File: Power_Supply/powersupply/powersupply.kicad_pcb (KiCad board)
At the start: 2 copper layers, 54 parts, among them J1 Conn_01x03, J2 USB_B_Micro, Q1 Q_PMOS_GDS, SW1 SW_Push, U1 AZ1117E-3.3, U10 MCP6001-OT, U2 ATSAMD10D13A-SS, U3 B0505S-2WR2, U4 TFT_OLED, U5 joystick-K1-1506DN-01, U6 MC33063AP1, U7 LM358P, U8 1x2, U9 1x2

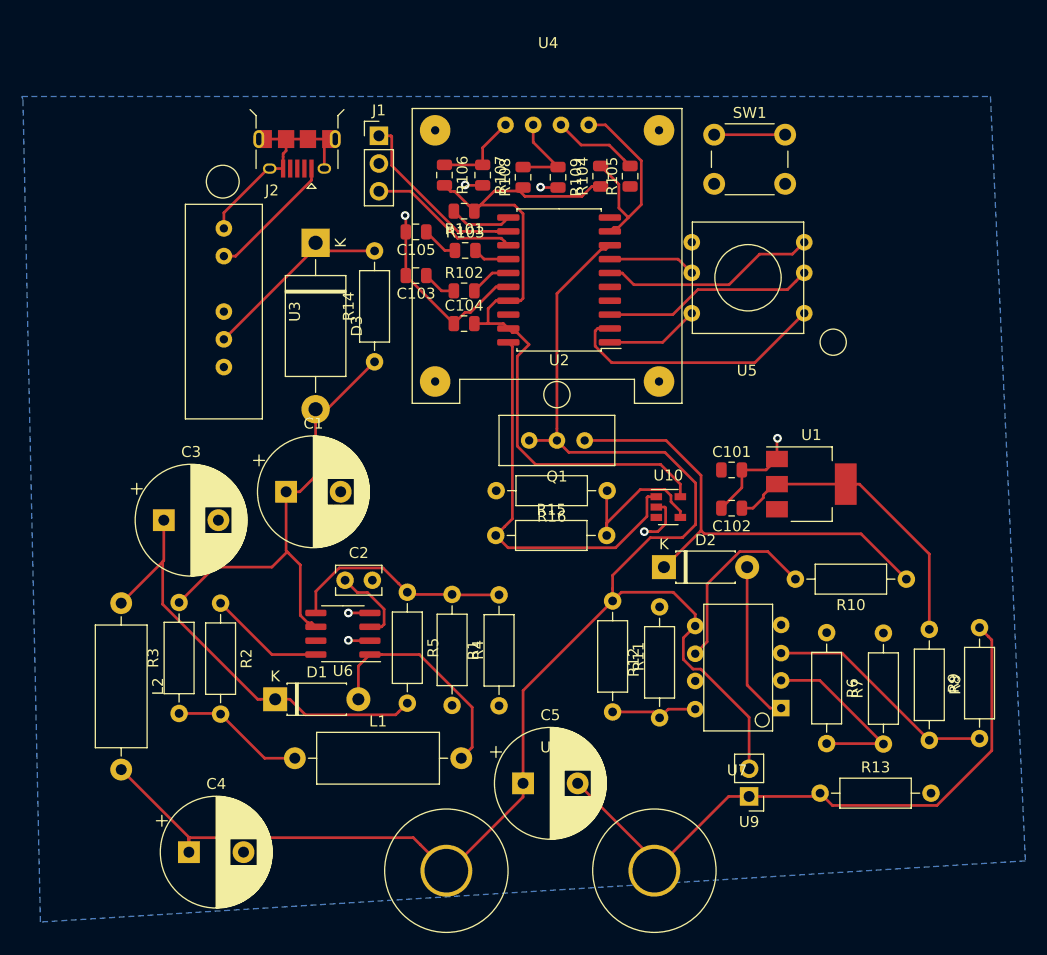
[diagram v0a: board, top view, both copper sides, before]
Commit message: layout changes
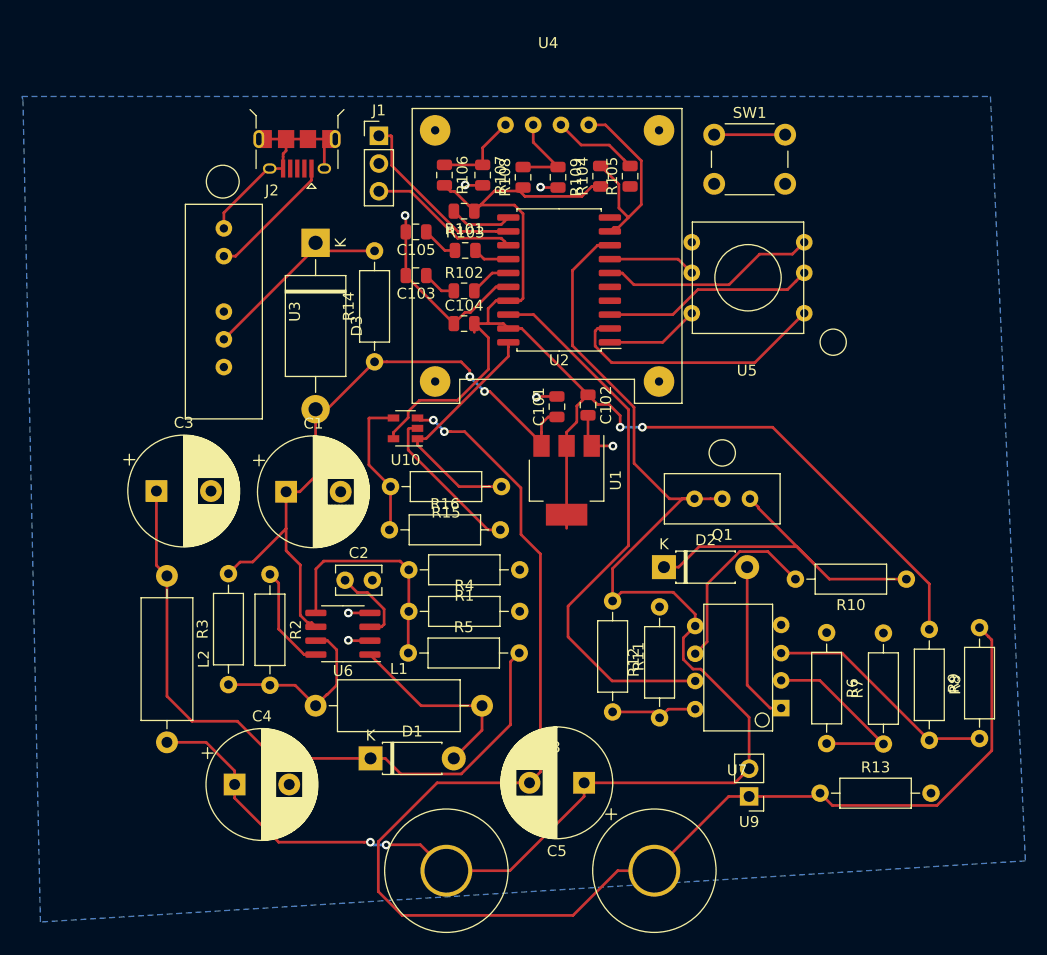
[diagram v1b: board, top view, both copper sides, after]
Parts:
- moved U10 25.1 mm to (75.1, 50.2), turned to 180 degrees
- moved U1 22.4 mm to (89.9, 54.9), turned to 270 degrees
- moved R16 20.3 mm to (73.7, 59.5), turned to 0 degrees
- moved C101 17.0 mm to (89.0, 48.2), turned to 90 degrees
- moved C102 16.2 mm to (91.8, 48.1), turned to 270 degrees
- moved Q1 16.1 mm to (104.1, 56.6)
- moved R1 12.6 mm to (85.6, 63.1), turned to 180 degrees
- moved D1 10.3 mm to (71.9, 80.4)
- moved C4 7.48 mm to (59.5, 82.8)
- moved C5 5.59 mm to (91.5, 82.7), turned to 180 degrees
- moved R5 5.57 mm to (75.4, 70.8), turned to 0 degrees
- moved R2 5.24 mm to (62.7, 63.6)
- moved R3 5.24 mm to (58.9, 73.7)
- moved L1 5.17 mm to (66.9, 75.6)
- moved L2 4.88 mm to (53.3, 63.7)
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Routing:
- net /V_negative_out: track 59.0 -> 137.0 mm, vias 0 -> 2
- net /V_lin_ctrl: track 0.00 -> 51.0 mm
- net +3V3: track 96.1 -> 122.2 mm, vias 0 -> 2
- net Net-(C3-Pad1): track 40.2 -> 62.4 mm
- net +5V: track 42.3 -> 60.0 mm, vias 0 -> 2
- net /V_current_amplified: track 36.6 -> 22.6 mm
- net Net-(D2-Pad1): track 42.5 -> 32.8 mm
- net /Boost_out: track 146.3 -> 137.4 mm, vias 0 -> 2
- net GND: track 39.9 -> 46.3 mm
- net Net-(L1-Pad1): track 12.3 -> 17.0 mm
- net Net-(D1-Pad2): track 21.0 -> 18.1 mm
- net Net-(R15-Pad2): track 15.0 -> 13.3 mm
- net Net-(R2-Pad1): track 10.7 -> 9.72 mm

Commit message: more layout
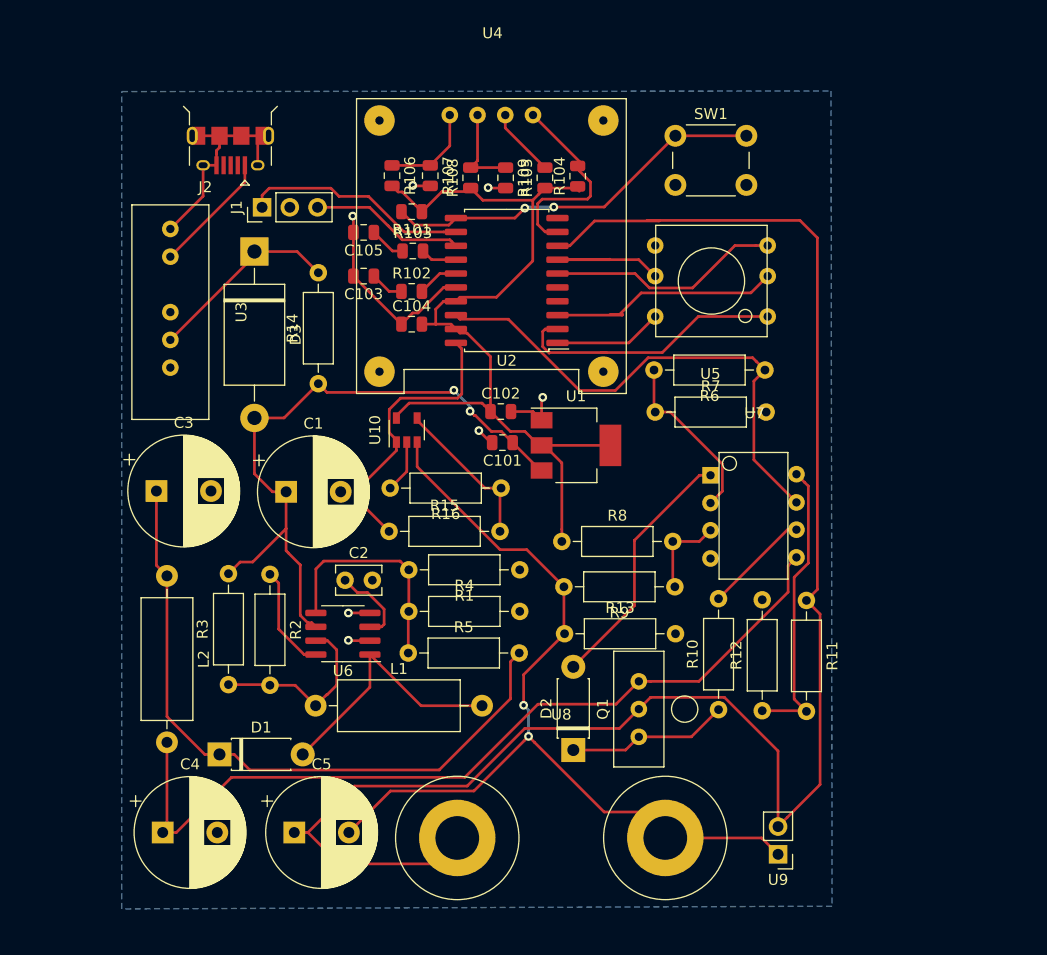
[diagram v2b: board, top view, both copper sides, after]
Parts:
- moved R7 36.9 mm to (98.0, 48.7), turned to 0 degrees
- moved R8 34.6 mm to (89.5, 60.5), turned to 0 degrees
- moved R9 31.2 mm to (99.8, 64.7), turned to 180 degrees
- moved R13 27.6 mm to (89.7, 69.0)
- moved C5 26.9 mm to (65.0, 87.2), turned to 0 degrees
- moved R6 24.7 mm to (108.0, 44.9), turned to 180 degrees
- moved R10 20.9 mm to (103.8, 76.0), turned to 90 degrees
- moved Q1 20.7 mm to (96.5, 75.9), turned to 90 degrees
- moved D2 18.7 mm to (90.5, 79.7), turned to 90 degrees
- moved R11 17.8 mm to (111.8, 66.0)
- moved U7 14.0 mm to (107.0, 58.2), turned to 0 degrees
- moved D1 13.8 mm to (58.1, 80.0)
- moved J1 12.5 mm to (62.0, 29.9), turned to 90 degrees
- moved R15 11.1 mm to (73.6, 59.6), turned to 0 degrees
- moved R16 10.9 mm to (83.9, 55.7), turned to 180 degrees
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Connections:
- C5 pad 1: /Boost_out -> /V_positive_out
- Q1 pad 2: /Boost_out -> /V_positive_out
- R11 pad 1: /Boost_out -> /V_positive_out
- R6 pad 1: /Vlim -> /V_lin_ctrl
- U2 pad 8: /Boost_out -> /V_positive_out
- U8 pad 2: /Boost_out -> /V_positive_out
- U9 pad 2: /Boost_out -> /V_positive_out
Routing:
- net /V_positive_out: track 0.00 -> 157.3 mm
- net /Boost_out: track 137.4 -> 78.3 mm, vias 2 -> 0
- net /V_negative_out: track 137.0 -> 83.2 mm
- net +3V3: track 122.2 -> 81.4 mm, vias 2 -> 0
- net Net-(R101-Pad2): track 12.3 -> 35.6 mm, vias 0 -> 2
- net Net-(R11-Pad2): track 8.12 -> 27.2 mm
- net Net-(D2-Pad1): track 32.8 -> 14.8 mm
- net Net-(R8-Pad2): track 21.5 -> 8.38 mm
- net GND: track 46.3 -> 37.1 mm
- net Net-(D2-Pad2): track 14.8 -> 23.3 mm
- net Net-(R10-Pad2): track 17.2 -> 9.75 mm
- net /right: track 8.02 -> 14.4 mm
- net Net-(D1-Pad2): track 18.1 -> 23.9 mm
- net /V_lin_ctrl: track 51.0 -> 47.0 mm
- net /SWCLK: track 17.0 -> 20.8 mm
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
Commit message: even more layout
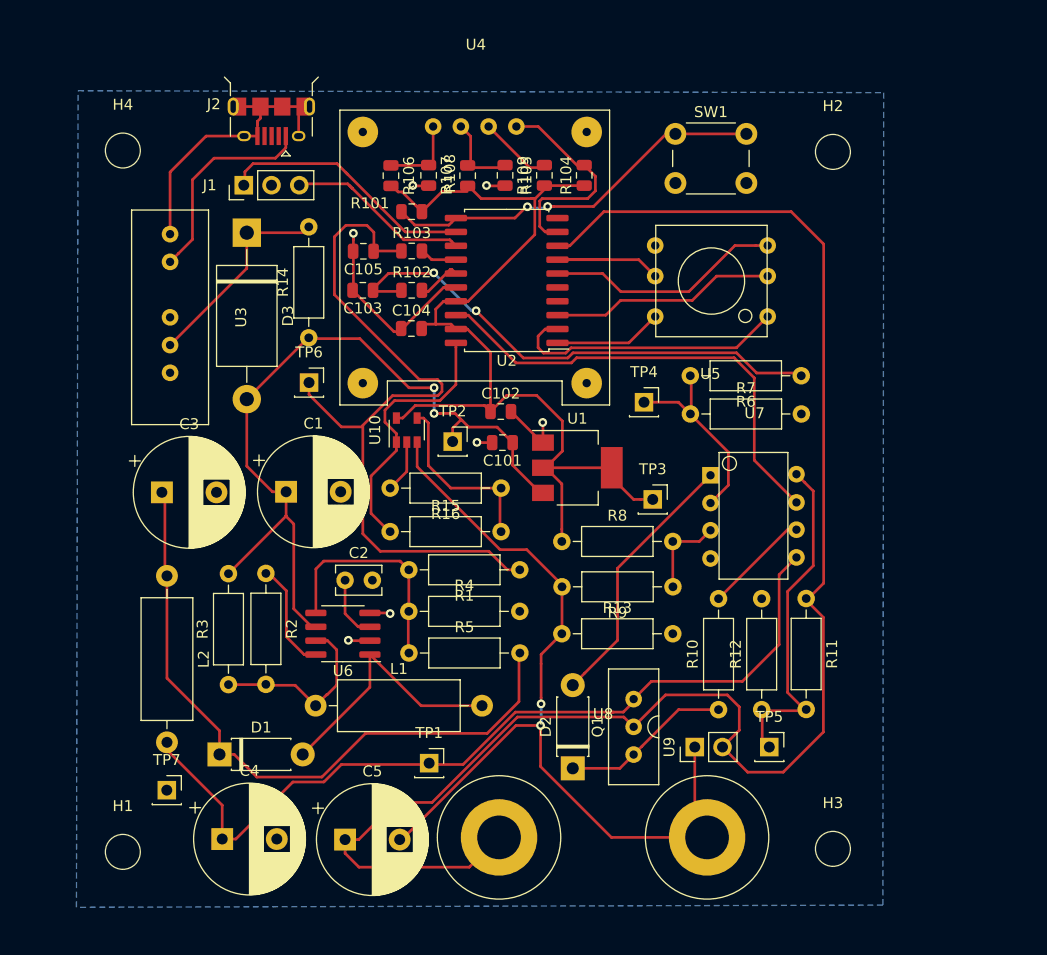
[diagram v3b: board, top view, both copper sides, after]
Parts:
- added H1: MountingHole, MountingHole:MountingHole_3.2mm_M3, F.Cu at (49.2, 89.0)
- added H2: MountingHole, MountingHole:MountingHole_3.2mm_M3, F.Cu at (114.3, 24.9)
- added H3: MountingHole, MountingHole:MountingHole_3.2mm_M3, F.Cu at (114.3, 88.7)
- added H4: MountingHole, MountingHole:MountingHole_3.2mm_M3, F.Cu at (49.2, 24.8)
- added TP1: Boost_out, Connector_PinSocket_2.54mm:PinSocket_1x01_P2.54mm_Vertical, F.Cu at (77.3, 80.8)
- added TP2: +5_isolated, Connector_PinSocket_2.54mm:PinSocket_1x01_P2.54mm_Vertical, F.Cu at (79.5, 51.4)
- added TP3: +3.3, Connector_PinSocket_2.54mm:PinSocket_1x01_P2.54mm_Vertical, F.Cu at (97.8, 56.7)
- added TP4: Current_limit, Connector_PinSocket_2.54mm:PinSocket_1x01_P2.54mm_Vertical, F.Cu at (97.0, 47.8)
- added TP5: Voltage_limit, Connector_PinSocket_2.54mm:PinSocket_1x01_P2.54mm_Vertical, F.Cu at (108.5, 79.4)
- added TP6: Boost_ctrl, Connector_PinSocket_2.54mm:PinSocket_1x01_P2.54mm_Vertical, F.Cu at (66.3, 46.0)
- added TP7: GND, Connector_PinSocket_2.54mm:PinSocket_1x01_P2.54mm_Vertical, F.Cu at (53.3, 83.3)
- moved U9 12.4 mm to (101.6, 79.4), turned to 90 degrees
- moved C4 5.48 mm to (58.4, 87.8)
- moved C5 4.70 mm to (69.6, 87.8)
- moved J2 4.61 mm to (62.9, 20.7)
- moved R14 4.29 mm to (66.3, 41.9)
- moved U8 3.83 mm to (93.2, 87.7)
- moved R6 3.37 mm to (111.4, 45.4)
- moved R7 3.23 mm to (101.2, 48.9)
- moved J1 2.63 mm to (60.3, 27.9)
- moved U1 2.05 mm to (90.9, 53.8)
- moved D3 1.86 mm to (60.6, 32.3)
- moved U4 1.85 mm to (81.5, 34.5)
- moved C105 1.73 mm to (71.3, 34.0)
- moved Q1 1.69 mm to (96.0, 77.5)
- moved D2 1.68 mm to (90.5, 81.3)
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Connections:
- net Net-(R11-Pad2) renamed /Voltage_limit_divider
- net Net-(R6-Pad2) renamed /Current_limit_divider
- R1 pad 1: /Vref -> /V_boost_ctrl
- R6 pad 1: /V_lin_ctrl -> /V_curr_lim
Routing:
- net /V_boost_ctrl: track 3.33 -> 69.2 mm
- net /V_curr_lim: track 3.10 -> 46.8 mm, vias 0 -> 2
- net +5V: track 60.7 -> 72.1 mm
- net +3V3: track 81.4 -> 91.4 mm
- net /V_positive_out: track 157.3 -> 148.7 mm
- net Net-(J2-Pad1): track 11.2 -> 19.2 mm
- net Net-(J2-Pad5): track 19.8 -> 26.7 mm
- net /Voltage_limit_divider: track 27.2 -> 31.5 mm
- net /V_lin_ctrl: track 47.0 -> 43.1 mm
- net /SWDIO: track 14.1 -> 17.1 mm
- net /Current_limit_divider: track 16.0 -> 18.8 mm
- net /SWCLK: track 20.8 -> 23.6 mm
- net Net-(R15-Pad2): track 14.5 -> 16.6 mm
- net /V_negative_out: track 83.2 -> 81.5 mm
- net Net-(C2-Pad1): track 7.46 -> 5.84 mm
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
